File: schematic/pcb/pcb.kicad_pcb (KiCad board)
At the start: 4 copper layers, 59.9 x 59.9 mm, 34 parts, among them J1 MAVLINK, J2 DISPLAY, J3 SER. SERVO, J4 MAG., J5 SERVO, J6 5V, P1 USB_C_Plug_USB2.0, Q1 NPN, Q2 NPN, U1 NEO-M9N

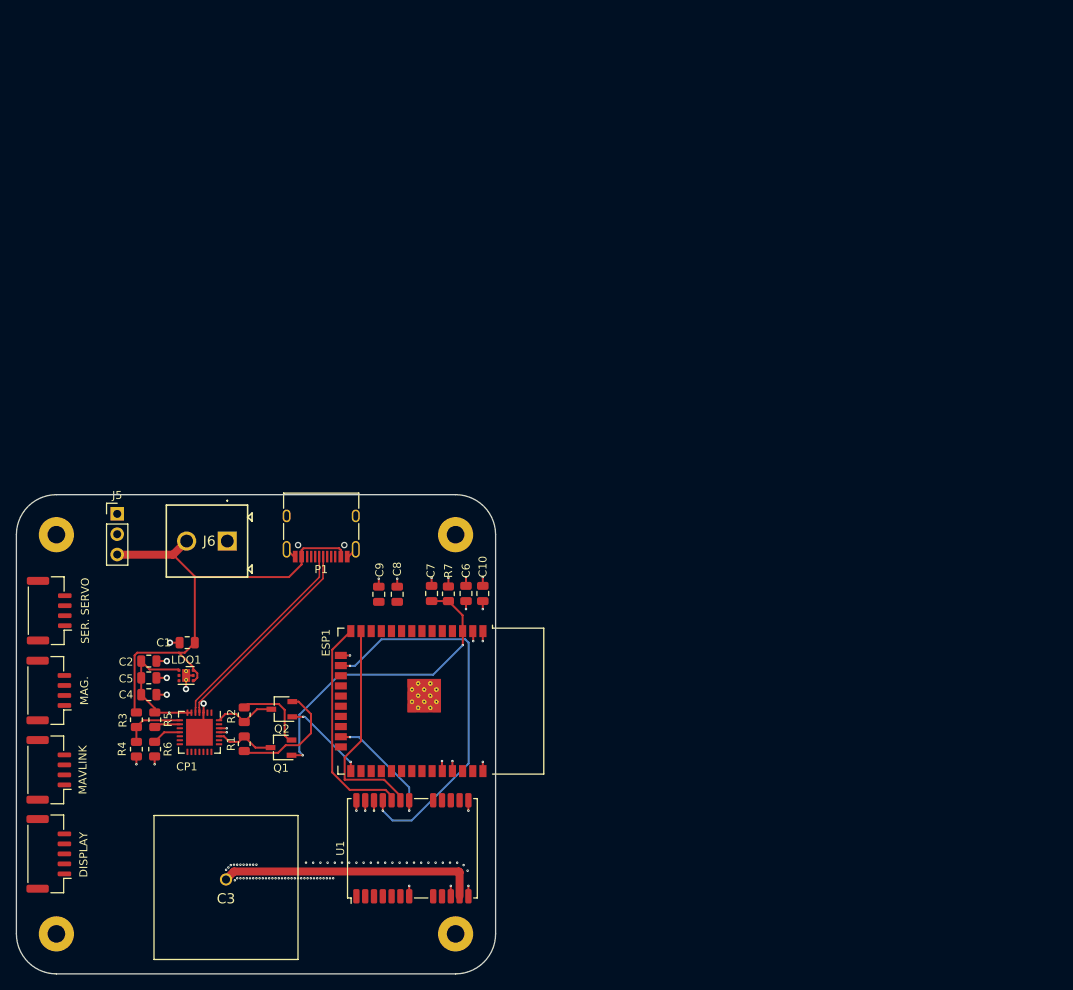
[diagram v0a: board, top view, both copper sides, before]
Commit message: new pcb
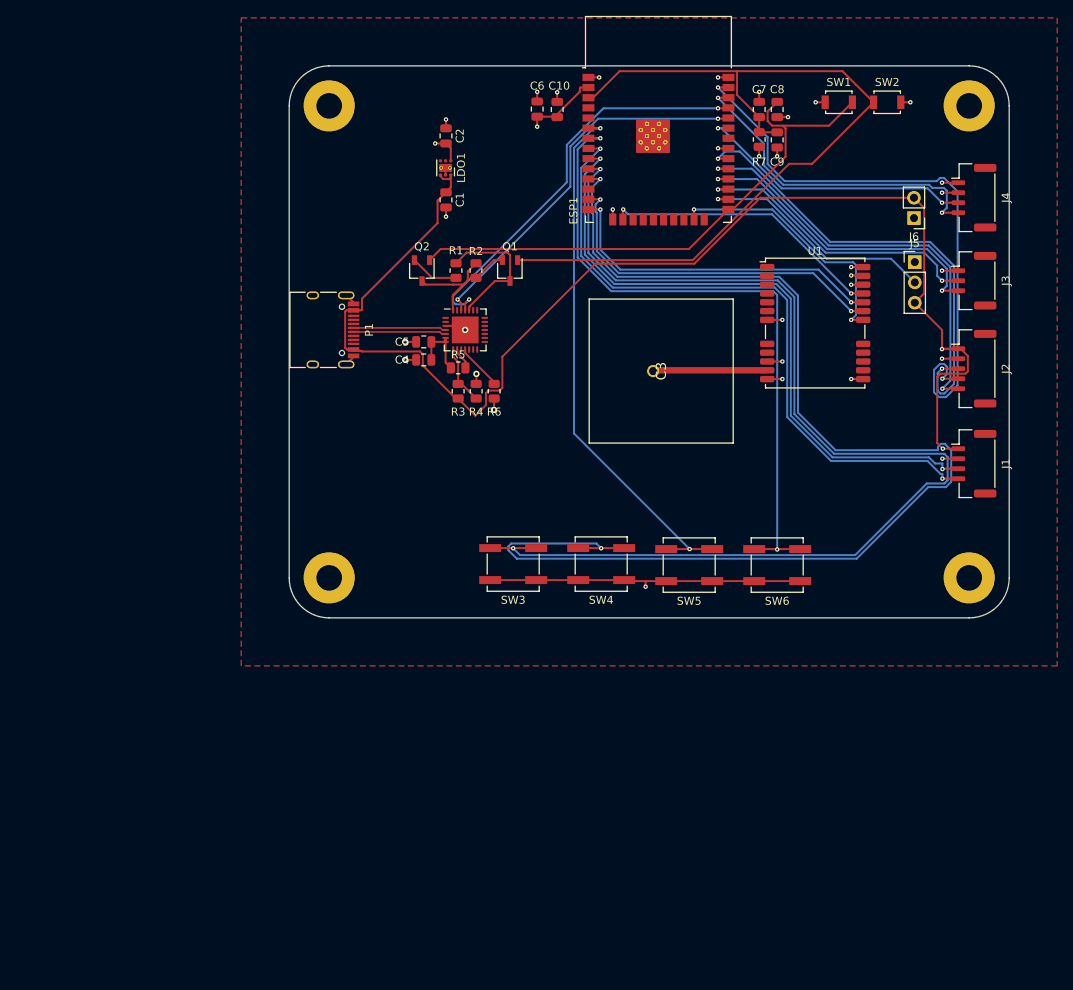
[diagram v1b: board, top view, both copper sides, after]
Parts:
- removed the REF** at (130.9, 88.6)
- removed the REF** at (180.8, 88.6)
- removed the REF** at (130.9, 138.5)
- removed the REF** at (180.8, 138.5)
- added ?: , , F.Cu at (245.0, 94.0)
- added ?: , , F.Cu at (165.0, 94.0)
- added REF**: MountingHole_3.2mm_M3_Pad, MountingHole:MountingHole_3.2mm_M3_Pad, F.Cu at (165.0, 35.0)
- added REF**: MountingHole_3.2mm_M3_Pad, MountingHole:MountingHole_3.2mm_M3_Pad, F.Cu at (245.0, 35.0)
- added SW1: SW_Push, Button_Switch_SMD:SW_SPST_B3U-1000P, F.Cu at (228.7, 34.5)
- added SW2: SW_Push, Button_Switch_SMD:SW_SPST_B3U-1000P, F.Cu at (234.8, 34.5)
- added SW3: SW_Push, Button_Switch_SMD:SW_SPST_B3SL-1002P, F.Cu at (188.0, 92.3)
- added SW4: SW_Push, Button_Switch_SMD:SW_SPST_B3SL-1002P, F.Cu at (199.0, 92.3)
- added SW5: SW_Push, Button_Switch_SMD:SW_SPST_B3SL-1002P, F.Cu at (210.0, 92.4)
- added SW6: SW_Push, Button_Switch_SMD:SW_SPST_B3SL-1002P, F.Cu at (221.0, 92.4)
- J3: footprint Connector_JST:JST_GH_BM04B-GHS-TBT_1x04-1MP_P1.25mm_Vertical -> Connector_JST:JST_GH_BM03B-GHS-TBT_1x03-1MP_P1.25mm_Vertical
- J6: footprint Connector_Amphenol:VI0221550000G -> Connector_PinHeader_2.54mm:PinHeader_1x02_P2.54mm_Vertical
- moved J4 131.0 mm to (245.6, 46.5), turned to -90 degrees
- moved J2 130.6 mm to (245.6, 67.8), turned to -90 degrees
- moved J3 122.7 mm to (245.6, 56.9), turned to -90 degrees
- moved J1 121.8 mm to (245.6, 79.7), turned to -90 degrees
- moved J5 104.6 mm to (238.2, 54.5)
- moved J6 94.9 mm to (238.1, 49.0)
- moved C3 83.0 mm to (205.5, 68.2), turned to -90 degrees
- moved U1 82.7 mm to (225.8, 62.1), turned to 0 degrees
- moved C8 77.0 mm to (221.0, 35.5), turned to 90 degrees
- moved ESP1 76.0 mm to (206.2, 39.7), turned to 0 degrees
- moved C9 75.5 mm to (221.0, 39.2), turned to 90 degrees
- moved C2 75.4 mm to (179.6, 38.8), turned to 90 degrees
- moved C7 73.1 mm to (218.8, 35.5)
- moved LDO1 71.3 mm to (179.6, 42.8), turned to -90 degrees
- moved R7 68.8 mm to (218.8, 39.2), turned to 90 degrees
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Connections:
- C1 pad 1: VBUS -> +5V
- ESP1 pad 10: unconnected-(ESP1-IO25-Pad10) -> BUTTON_1
- ESP1 pad 11: unconnected-(ESP1-IO26-Pad11) -> BUTTON_2
- ESP1 pad 26: unconnected-(ESP1-IO4-Pad26) -> SERVO
- ESP1 pad 27: unconnected-(ESP1-IO16-Pad27) -> SERVO_RX
- ESP1 pad 28: unconnected-(ESP1-IO17-Pad28) -> SERVO_TX
- ESP1 pad 33: unconnected-(ESP1-IO21-Pad33) -> MAG_SDI
- ESP1 pad 36: unconnected-(ESP1-IO22-Pad36) -> MAG_SCK
- ESP1 pad 6: unconnected-(ESP1-IO34-Pad6) -> BUTTON_3
- ESP1 pad 7: unconnected-(ESP1-IO35-Pad7) -> BUTTON_4
- ESP1 pad 8: unconnected-(ESP1-IO32-Pad8) -> MAV_TX
- ESP1 pad 9: unconnected-(ESP1-IO33-Pad9) -> MAV_RX
- J1 pad 1: unconnected-(J1-Pin_1-Pad1) -> +5V
- J1 pad 2: unconnected-(J1-Pin_2-Pad2) -> GND
- J1 pad 3: unconnected-(J1-Pin_3-Pad3) -> MAV_RX
- J1 pad 4: unconnected-(J1-Pin_4-Pad4) -> MAV_TX
- J2 pad 1: unconnected-(J2-Pin_1-Pad1) -> +5V
- J2 pad 2: unconnected-(J2-Pin_2-Pad2) -> GND
- J2 pad 3: unconnected-(J2-Pin_3-Pad3) -> SCREEN_SCK
- J2 pad 4: unconnected-(J2-Pin_4-Pad4) -> SCREEN_MOSI
- J2 pad 5: unconnected-(J2-Pin_5-Pad5) -> SCREEN_CS
- J3 pad 1: unconnected-(J3-Pin_1-Pad1) -> GND
- J3 pad 2: unconnected-(J3-Pin_2-Pad2) -> SERVO_RX
- J3 pad 3: unconnected-(J3-Pin_3-Pad3) -> SERVO_TX
- J4 pad 1: unconnected-(J4-Pin_1-Pad1) -> +3V3
- J4 pad 2: unconnected-(J4-Pin_2-Pad2) -> GND
- J4 pad 3: unconnected-(J4-Pin_3-Pad3) -> MAG_SDI
- J4 pad 4: unconnected-(J4-Pin_4-Pad4) -> MAG_SCK
- J5 pad 2: unconnected-(J5-Pin_2-Pad2) -> SERVO
- J5 pad 3: VBUS -> +5V
- J6 pad 2: VBUS -> +5V
- LDO1 pad 4: VBUS -> +5V
- LDO1 pad 6: VBUS -> +5V
- P1 pad A4: VBUS -> +5V
- P1 pad A9: VBUS -> +5V
- P1 pad B4: VBUS -> +5V
- P1 pad B9: VBUS -> +5V
- R3 pad 1: VBUS -> +5V
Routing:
- net +5V: track 0.00 -> 164.4 mm, vias 0 -> 2
- net BUTTON_2: track 0.00 -> 157.6 mm, vias 0 -> 2
- net BUTTON_1: track 0.00 -> 143.9 mm, vias 0 -> 2
- net MAV_TX: track 0.00 -> 83.5 mm, vias 0 -> 2
- net BUTTON_4: track 0.00 -> 82.9 mm, vias 0 -> 2
- net MAV_RX: track 0.00 -> 81.1 mm, vias 0 -> 2
- net SCREEN_MOSI: track 0.00 -> 75.6 mm, vias 0 -> 2
- net BUTTON_3: track 0.00 -> 67.7 mm, vias 0 -> 2
- net VBUS: track 63.5 -> 0.00 mm
- net EN: track 39.0 -> 102.3 mm, vias 2 -> 0
- net SCREEN_SCK: track 0.00 -> 59.6 mm, vias 0 -> 2
- net IO0: track 10.8 -> 68.8 mm, vias 2 -> 0
- net SCREEN_CS: track 0.00 -> 53.1 mm, vias 0 -> 2
- net GND: track 31.1 -> 83.2 mm, vias 88 -> 27
- net MAG_SCK: track 0.00 -> 41.4 mm, vias 0 -> 2
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- added copper zone on F.Cu, net GND
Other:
- board size 59.9 x 59.9 mm -> 90 x 69 mm
